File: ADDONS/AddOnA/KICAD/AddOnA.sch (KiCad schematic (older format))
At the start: 55 parts, among them IC1 FIN1002, IC101 74HC251, IC6 PCA9536D, P1 10K0, SW1 Switch_DPDT, SW2 Switch_DPDT, X1 RCA, X101 XLR3, X110 PLR135_T10, X114 CON_IDC26, X115 CON_IDC26, X2 XLR3, X3 RCA, X4 Conn_01x03, X5 MicroMatch14, X6 HDR_02x08, X7 PLT133_T10W, X8 CON_USB_B, X9 USB_A

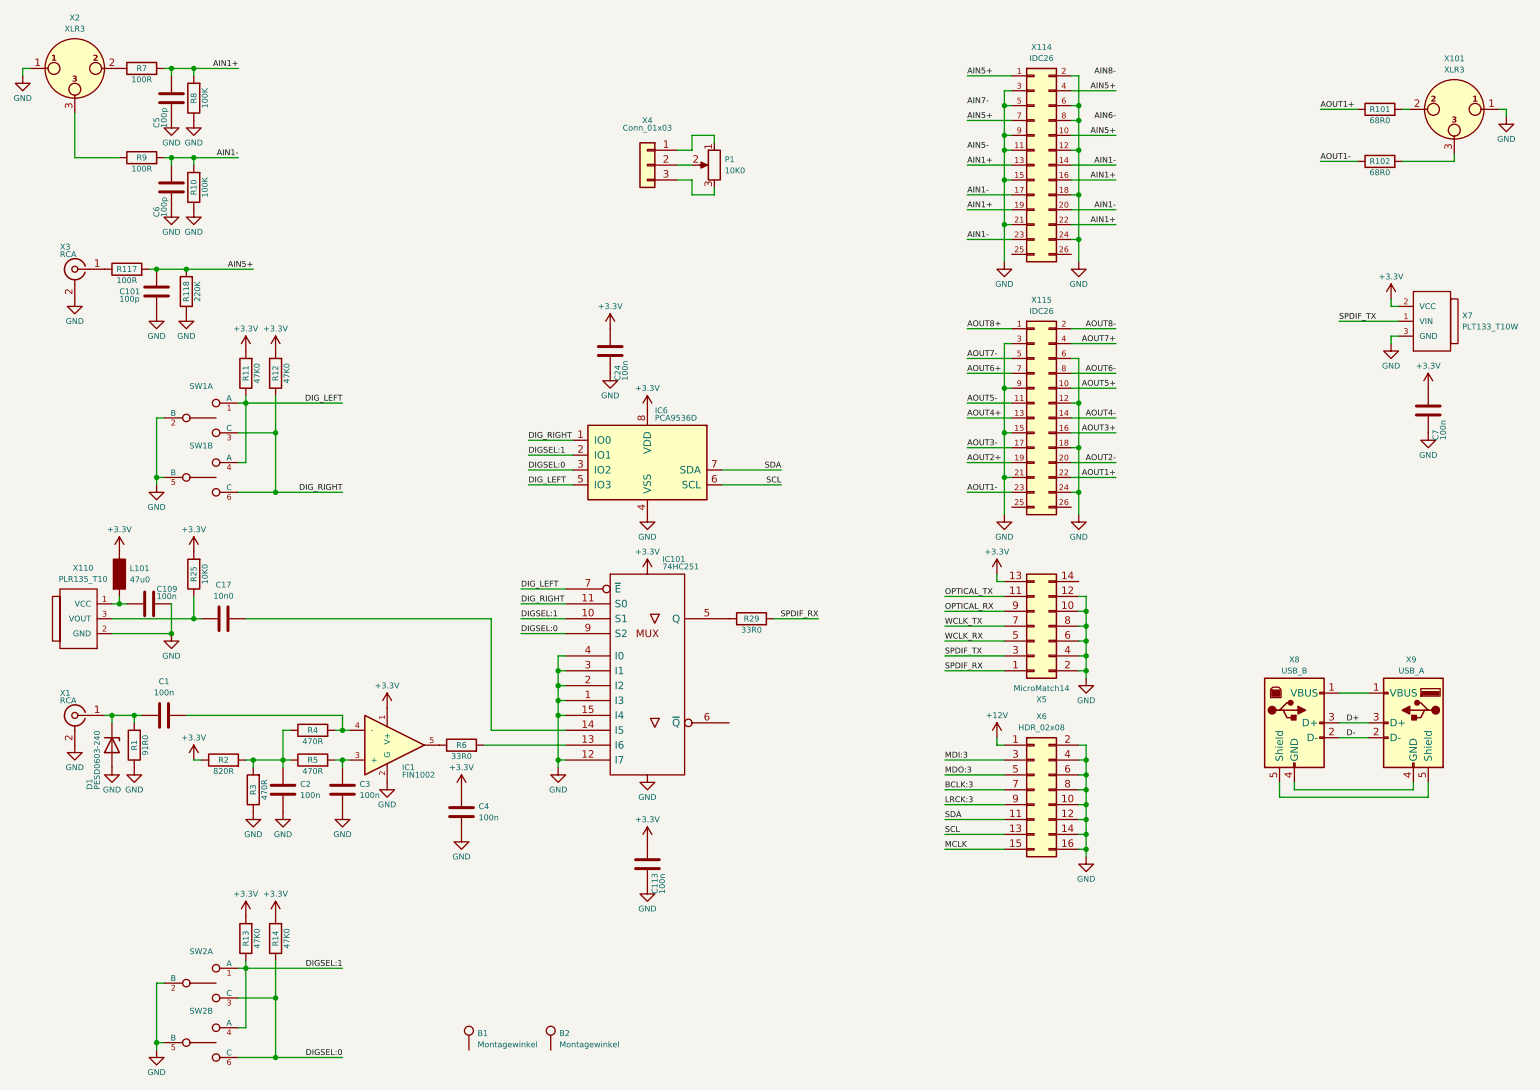
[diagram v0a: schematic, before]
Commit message: Updated Gerbers
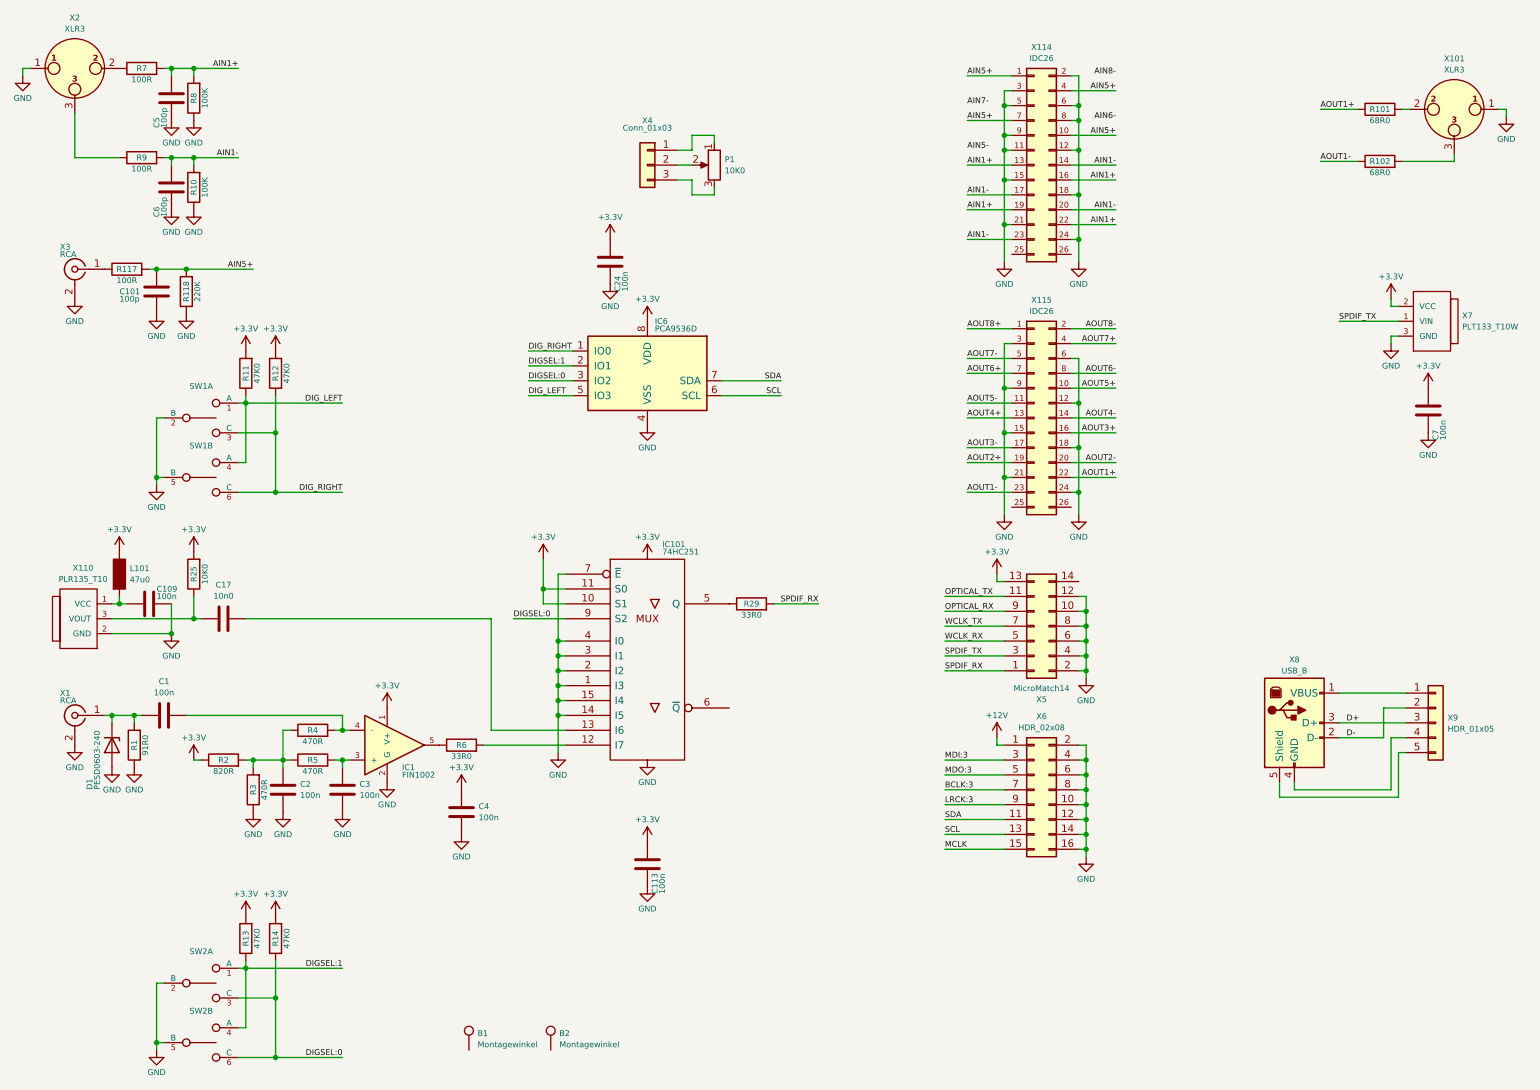
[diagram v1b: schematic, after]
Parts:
- removed X9: USB_A, Connector_USB:USB_A_CNCTech_1001-011-01101_Horizontal, symbol Connector:USB_A
- added X9: HDR_01x05, Connector_PinHeader_2.54mm:PinHeader_1x05_P2.54mm_Vertical, symbol Connector_Generic:Conn_01x05
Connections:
- net +3V3: now also IC101.10 (S1), IC101.11 (S0)
- net D+: now also X9.3 (Pin_3)
- net D-: now also X9.2 (Pin_2)
- net DIGSEL:1: no longer IC101.10 (S1)
- net DIG_LEFT: no longer IC101.7 (~E)
- net DIG_RIGHT: no longer IC101.11 (S0)
- net GND: now also IC101.14 (I5), IC101.7 (~E); no longer IC101.12 (I7)
- net at R6.2: now also IC101.12 (I7); no longer IC101.13 (I6)
- net at C17.2: now also IC101.13 (I6); no longer IC101.14 (I5)
- net at X8.1 (VBUS): now also X9.1 (Pin_1)
- net at X8.4 (GND): now also X9.4 (Pin_4)
- net at X8.5 (Shield): now also X9.5 (Pin_5)
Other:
- moved on the sheet: C24, IC101, IC6, R29
